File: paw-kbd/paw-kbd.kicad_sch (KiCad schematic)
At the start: 46 parts, among them J1 OLED, J2 MJ-4PP-9, SW1 SW_PUSH, SW10 SW_PUSH, SW11 SW_PUSH, SW12 SW_PUSH, SW13 SW_PUSH, SW14 SW_PUSH, SW15 SW_PUSH, SW16 SW_PUSH, SW17 SW_PUSH, SW2 SW_PUSH, SW3 SW_PUSH, SW4 SW_PUSH, SW5 SW_PUSH, SW6 SW_PUSH, SW7 SW_PUSH, SW8 SW_PUSH, SW9 SW_PUSH, U1 ProMicro

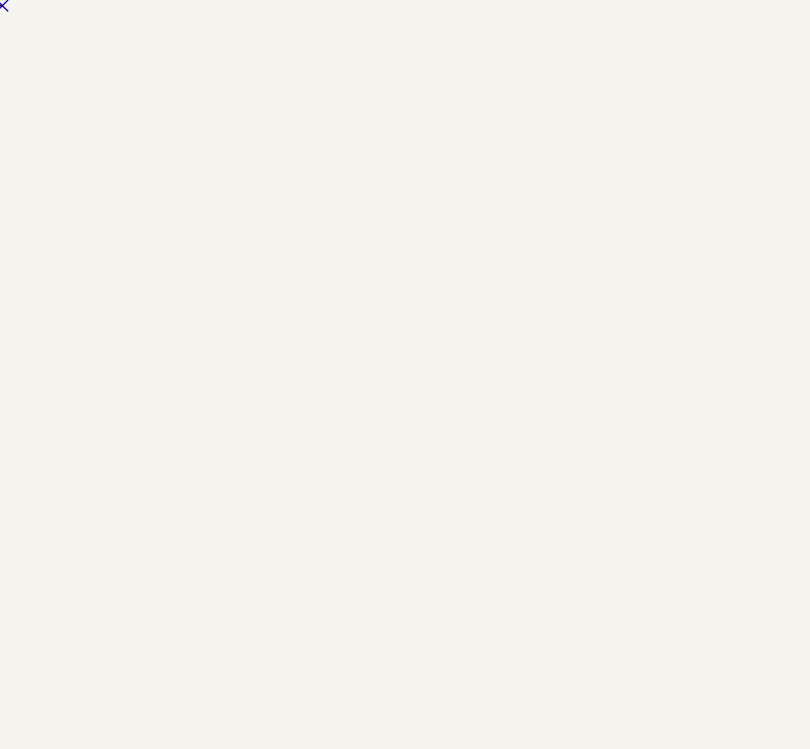
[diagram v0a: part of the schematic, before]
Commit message: wip
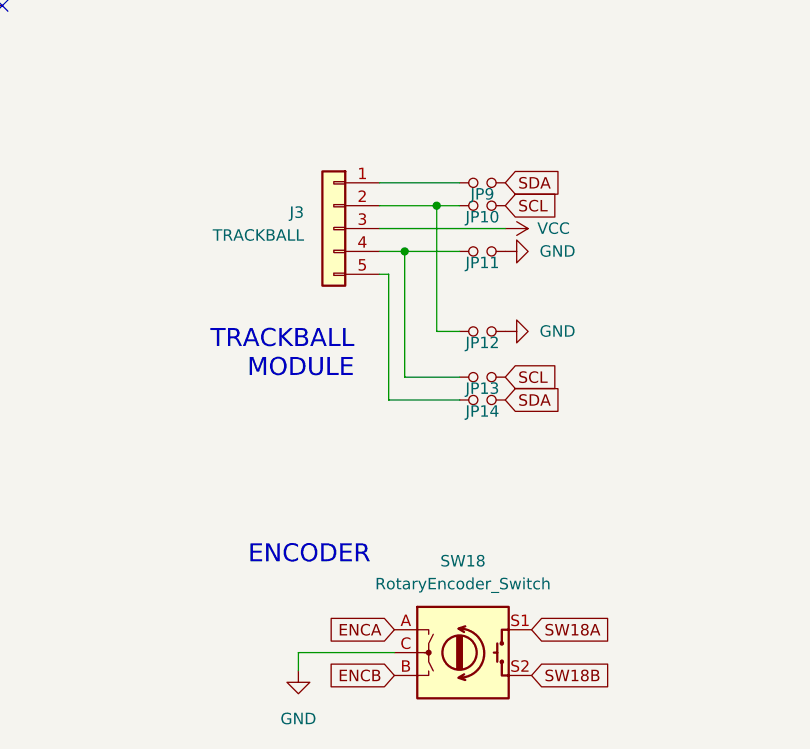
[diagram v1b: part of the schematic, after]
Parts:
- added J3: TRACKBALL, keeb-footprints:pimoroni, symbol Connector_Generic:Conn_01x05
- added JP10, JP11, JP12, JP14, JP9: Device_Jumper_NO_Small, kbd:Jumper, symbol KLORlib:Device_Jumper_NO_Small
- added JP13: Device_Jumper_NO_Small, kbd:Jumper, symbol SofleKeyboard-cache:Device_Jumper_NO_Small
- added SW18: RotaryEncoder_Switch, Rotary_Encoder:RotaryEncoder_Alps_EC12E-Switch_Vertical_H20mm, symbol Device:RotaryEncoder_Switch
- J1: footprint kbd:OLED_v2 -> keeb-footprints:SSD1306_128x64OLED
- U1: footprint keeb-footprints:ProMicro_unrouted_type_c -> keeb-footprints:ProMicro_v2
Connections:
- net GND: now also JP11.2, JP12.2, SW18.C
- net SCL: now also JP10.2, JP13.2
- net SDA: now also JP14.2, JP9.2
- net VCC: now also J3.3 (Pin_3)
- new net: J3.2 (Pin_2), JP10.1, JP12.1
- new net: J3.1 (Pin_1), JP9.1
- new net: J3.4 (Pin_4), JP11.1, JP13.1
- new net: J3.5 (Pin_5), JP14.1
- new net ENCA: SW18.A
- new net ENCB: SW18.B
- new net SW18A: SW18.S1
- new net SW18B: SW18.S2
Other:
- note added: "ENCODER"
- note added: "TRACKBALL MODULE"
